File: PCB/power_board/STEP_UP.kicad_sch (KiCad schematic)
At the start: 23 parts, among them IC1 TPS6213013AQRGTTQ1, IC11 TPS61032PWP, IC8 TPS63000IDRCRQ1

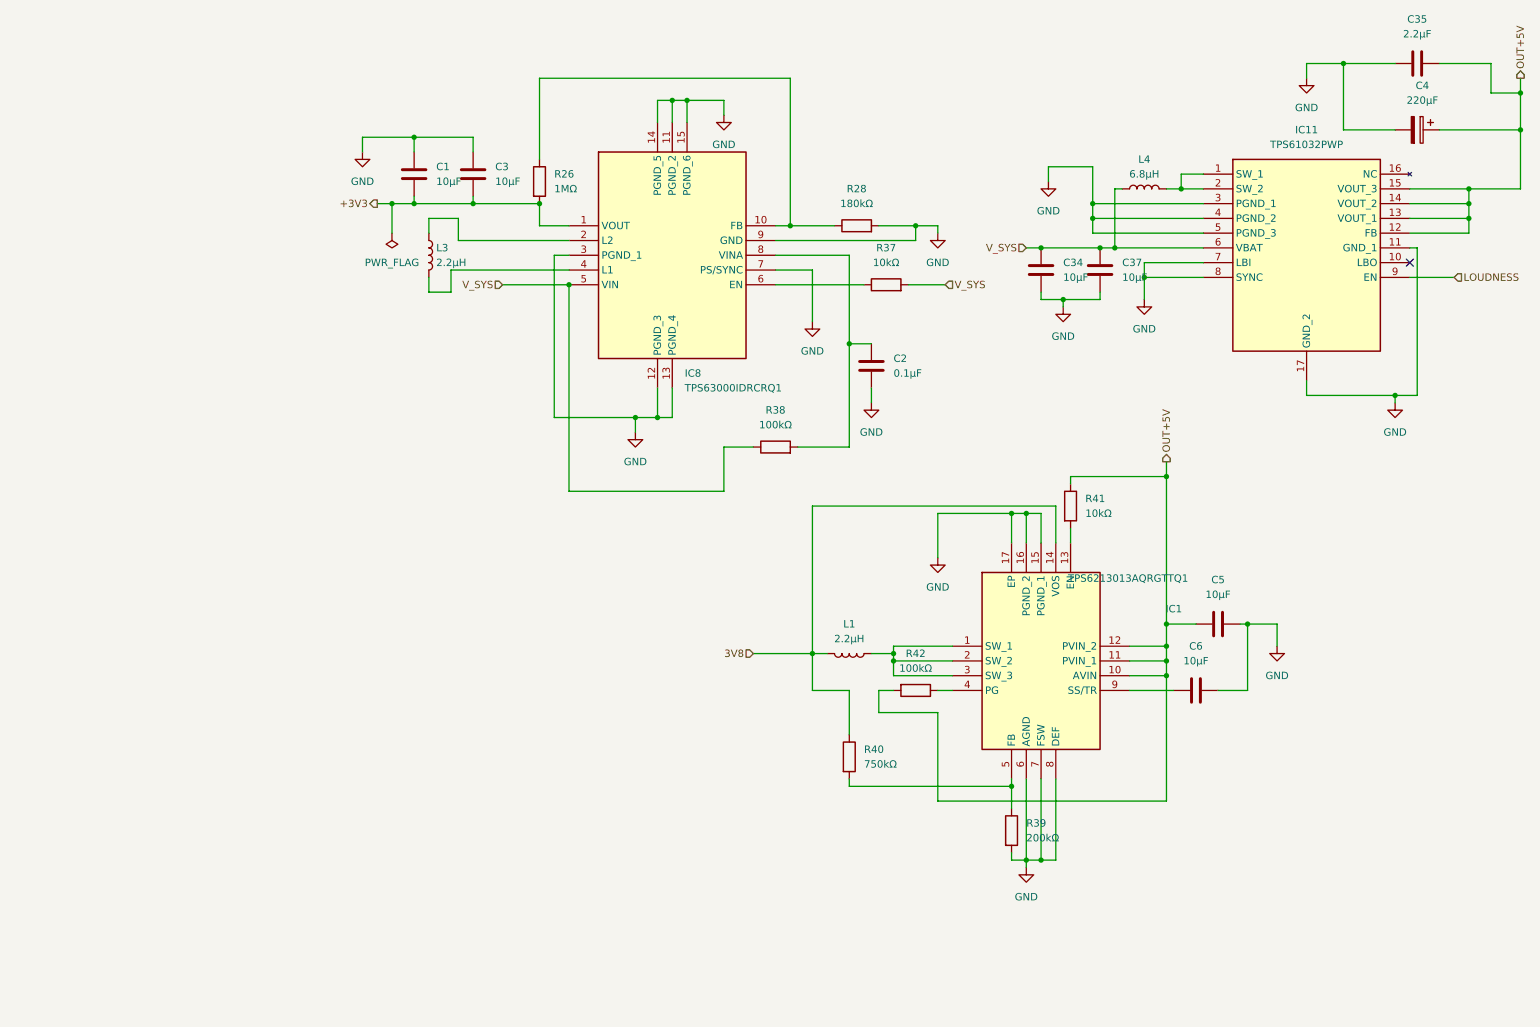
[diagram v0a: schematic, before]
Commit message: imu from board
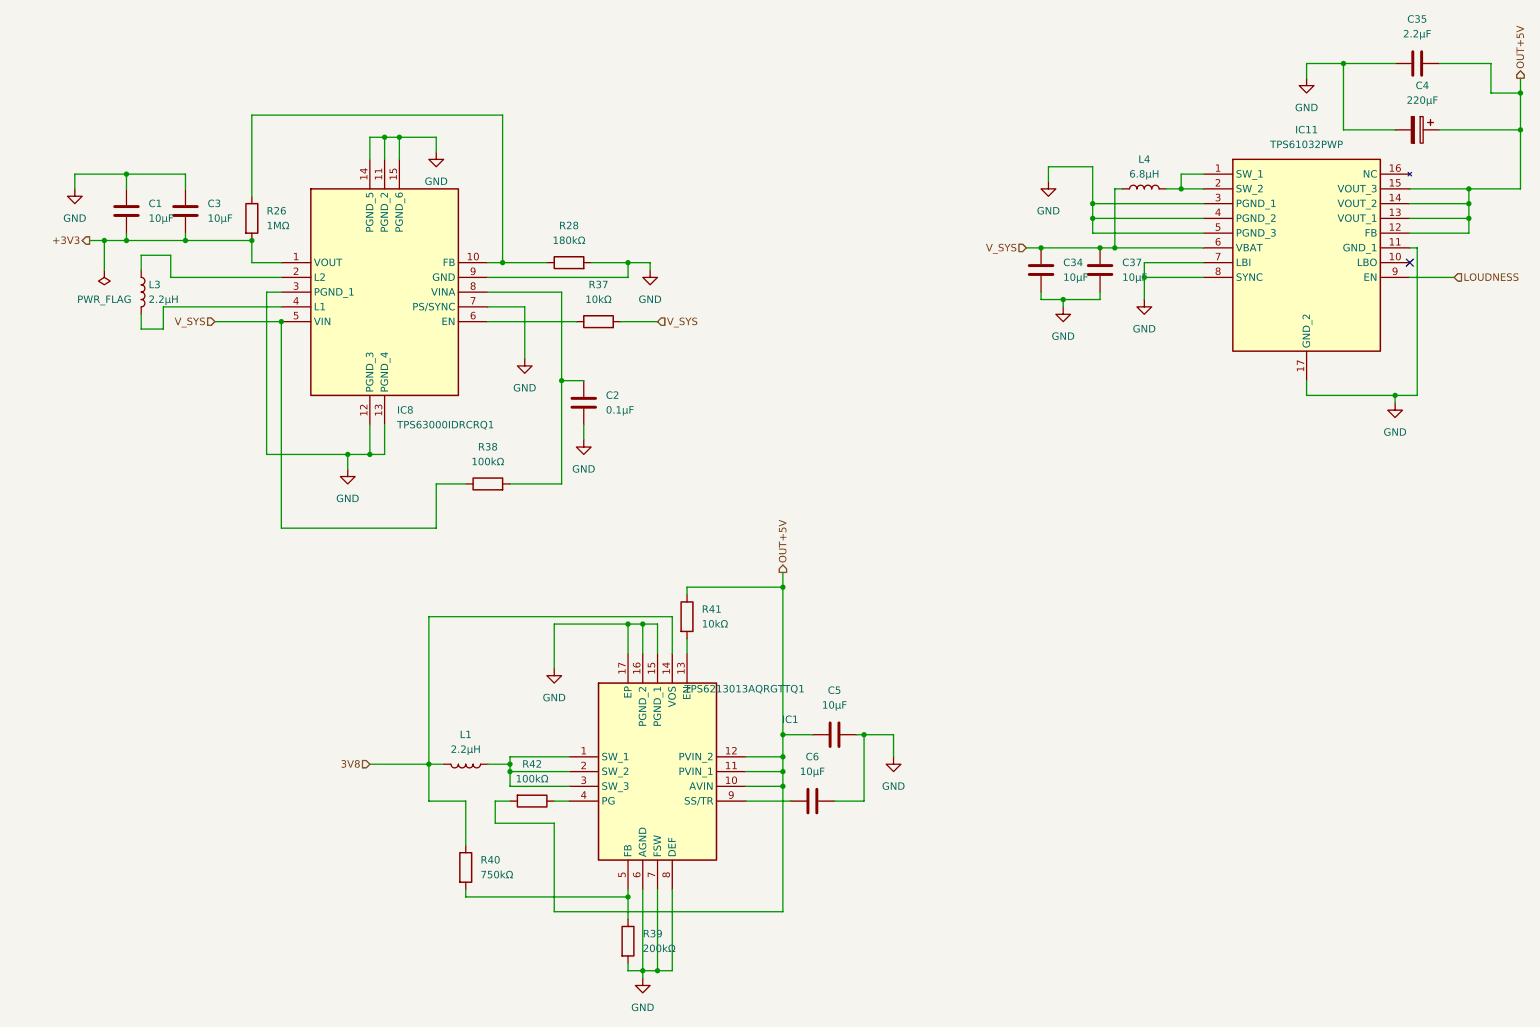
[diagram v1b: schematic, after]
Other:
- moved on the sheet: C1, C2, C3, C5, C6, IC1, IC8, L1, L3, R26, R28, R37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

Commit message: before smd
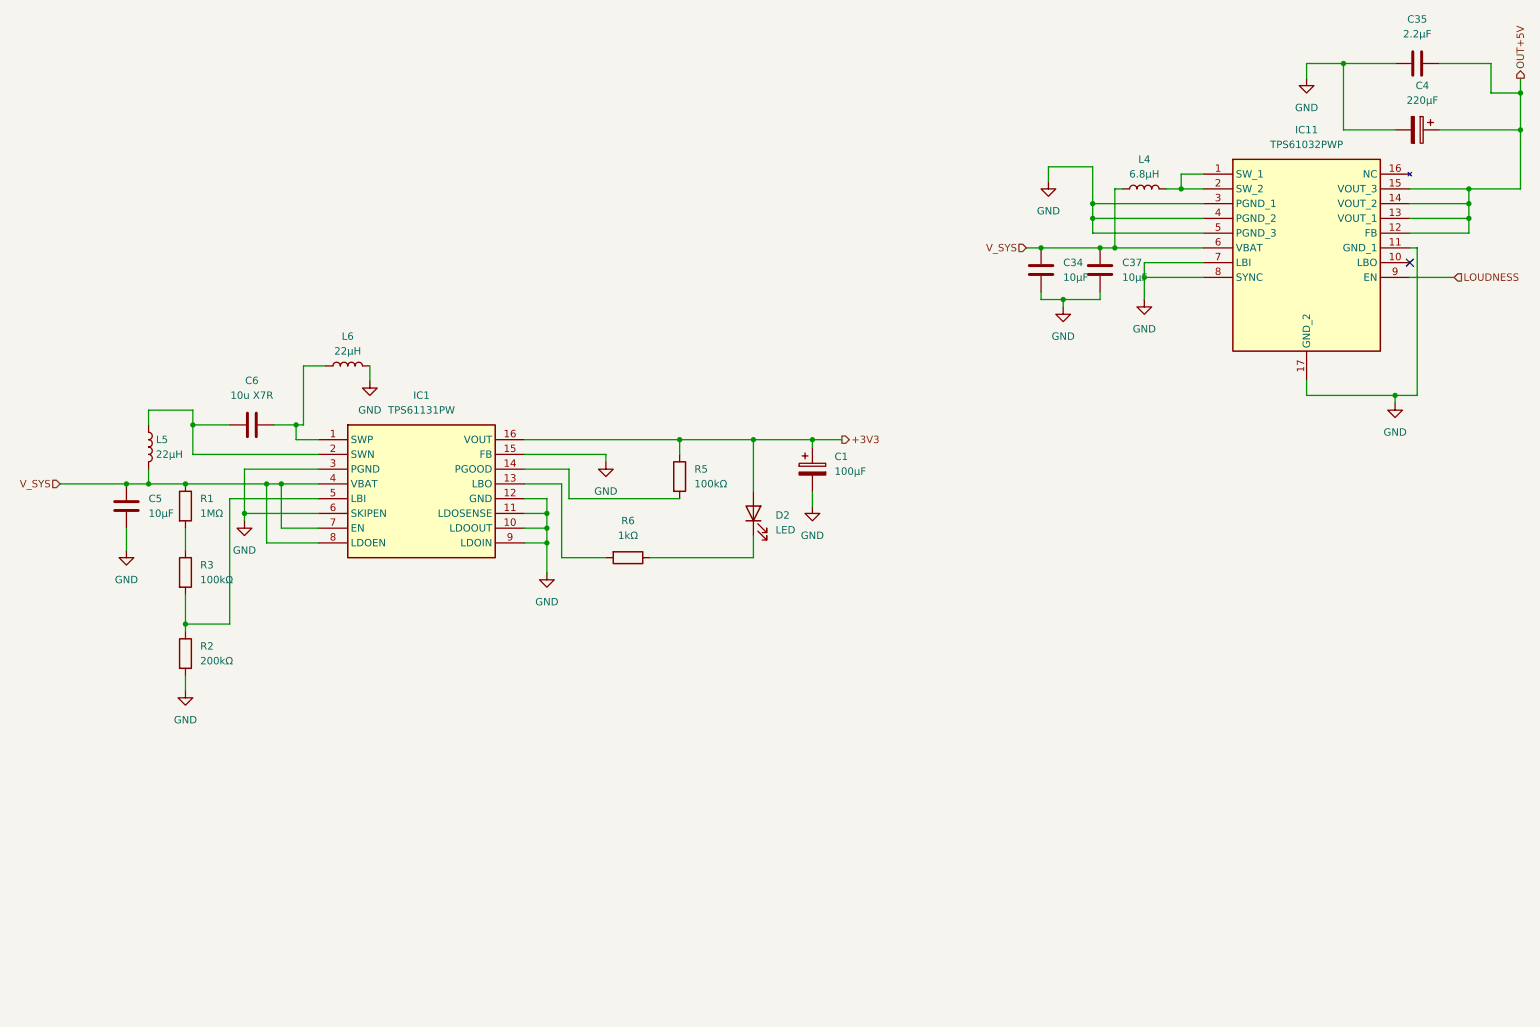
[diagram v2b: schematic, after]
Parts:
- removed C1, C3: 10μF, Capacitor_THT:C_Disc_D5.0mm_W2.5mm_P2.50mm, symbol Device:C
- removed C2: 0.1μF, Capacitor_THT:C_Disc_D5.0mm_W2.5mm_P2.50mm, symbol Device:C
- removed IC1: TPS6213013AQRGTTQ1, TPS6213013AQRGTTQ1:QFN50P300X300X100-17N-D, symbol TPS6213013AQRGTTQ1:TPS6213013AQRGTTQ1
- removed IC8: TPS63000IDRCRQ1, TPS63000IDRCRQ1:TPS63000IDRCRQ1, symbol TPS63000IDRCRQ1:TPS63000IDRCRQ1
- removed L1, L3: 2.2µH, Inductor_THT:L_Axial_L7.0mm_D3.3mm_P10.16mm_Horizontal_Fastron_MICC, symbol Device:L
- removed R26: 1MΩ, Resistor_THT:R_Axial_DIN0207_L6.3mm_D2.5mm_P7.62mm_Horizontal, symbol Device:R
- removed R28: 180kΩ, Resistor_THT:R_Axial_DIN0207_L6.3mm_D2.5mm_P7.62mm_Horizontal, symbol Device:R
- removed R37, R41: 10kΩ, Resistor_THT:R_Axial_DIN0207_L6.3mm_D2.5mm_P7.62mm_Horizontal, symbol Device:R
- removed R38, R42: 100kΩ, Resistor_THT:R_Axial_DIN0207_L6.3mm_D2.5mm_P7.62mm_Horizontal, symbol Device:R
- removed R39: 200kΩ, Resistor_THT:R_Axial_DIN0207_L6.3mm_D2.5mm_P7.62mm_Horizontal, symbol Device:R
- removed R40: 750kΩ, Resistor_THT:R_Axial_DIN0207_L6.3mm_D2.5mm_P7.62mm_Horizontal, symbol Device:R
- added C1: 100μF, Capacitor_Tantalum_SMD:CP_EIA-3216-18_Kemet-A, symbol Device:C_Polarized
- added D2: LED, LED_SMD:LED_0603_1608Metric, symbol Device:LED
- added IC1: TPS61131PW, TPS61131PW:SOP65P640X120-16N, symbol TPS61131PW:TPS61131PW
- added L5: 22µH, Inductor_SMD:L_6.3x6.3_H3, symbol Device:L
- added L6: 22µH, Inductor_THT:L_Axial_L7.0mm_D3.3mm_P10.16mm_Horizontal_Fastron_MICC, symbol Device:L
- added R1: 1MΩ, Resistor_SMD:R_0603_1608Metric, symbol Device:R
- added R2: 200kΩ, Resistor_SMD:R_0603_1608Metric, symbol Device:R
- added R3, R5: 100kΩ, Resistor_SMD:R_0603_1608Metric, symbol Device:R
- added R6: 1kΩ, Resistor_SMD:R_0603_1608Metric, symbol Device:R
- C34, C35, C37, C4: footprint Capacitor_THT:C_Disc_D5.0mm_W2.5mm_P2.50mm -> Capacitor_SMD:CP_Elec_6.3x5.4
- C5: value 10µF -> 10μF; footprint Capacitor_THT:C_Disc_D5.0mm_W2.5mm_P2.50mm -> Capacitor_SMD:CP_Elec_6.3x5.4
- C6: value 10µF -> 10u X7R; footprint Capacitor_THT:C_Disc_D5.0mm_W2.5mm_P2.50mm -> Capacitor_SMD:CP_Elec_6.3x5.4
- L4: footprint Inductor_THT:L_Axial_L7.0mm_D3.3mm_P10.16mm_Horizontal_Fastron_MICC -> Inductor_SMD:L_6.3x6.3_H3
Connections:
- net +3V3: now also C1.1, D2.2 (A), IC1.16 (VOUT), R5.1
- net GND: now also C5.2, C1.2, IC1.10 (LDOOUT), IC1.11 (LDOSENSE), IC1.12 (GND), IC1.15 (FB), IC1.3 (PGND), IC1.6 (SKIPEN), IC1.9 (LDOIN), L6.2, R2.2; no longer C5.1, C6.1
- net OUT+5V: no longer C5.2
- net V_SYS: now also C5.1, IC1.4 (VBAT), IC1.7 (EN), IC1.8 (LDOEN), L5.2, R1.1
- net at C6.2: now also IC1.2 (SWN), L5.1
- new net: R1.2, R3.1
- new net: C6.1, IC1.1 (SWP), L6.1
- new net: IC1.13 (LBO), R6.2
- new net: IC1.14 (PGOOD), R5.2
- new net: IC1.5 (LBI), R2.1, R3.2
- new net: D2.1 (K), R6.1
